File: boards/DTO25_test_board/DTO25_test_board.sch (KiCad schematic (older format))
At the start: 9 parts, among them J1 MicroFit_11, J2 Ultrafit_4, J3 Ultrafit_2, J4 Ultrafit_4

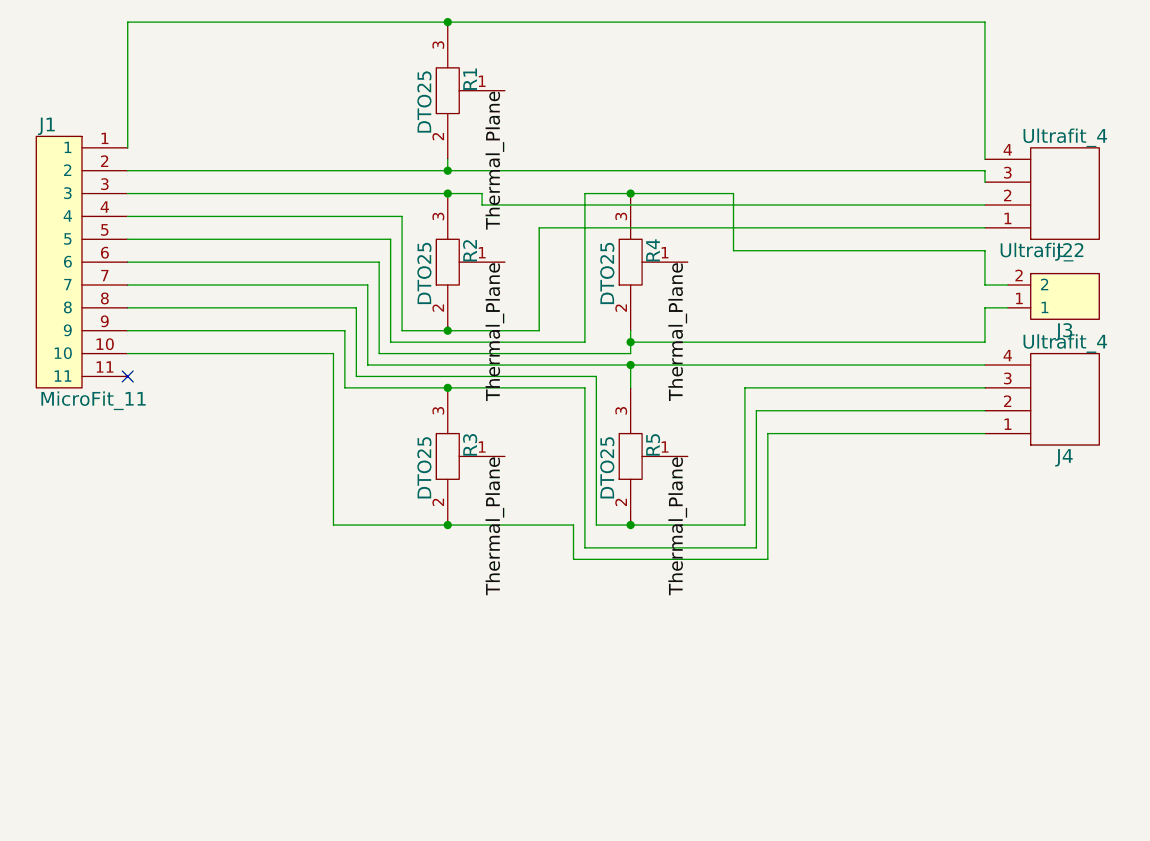
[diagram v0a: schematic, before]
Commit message: DTO@% test board MKII
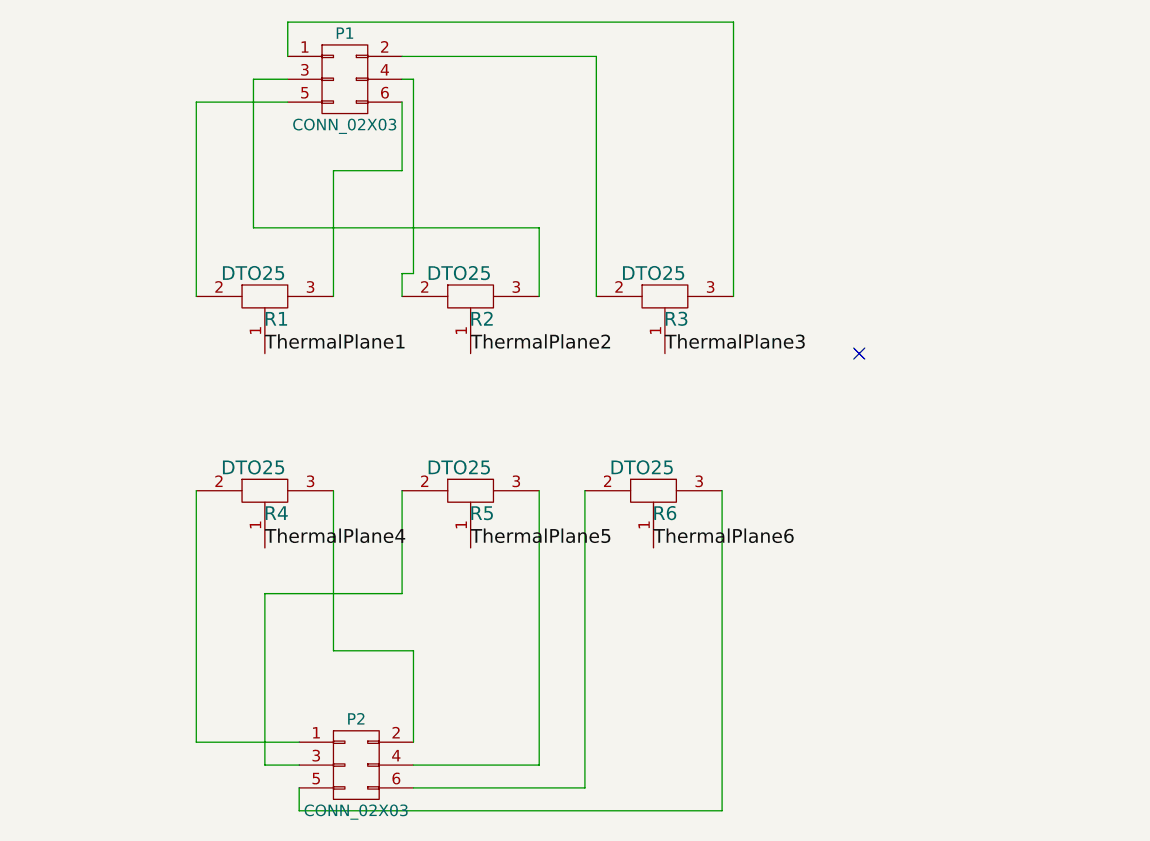
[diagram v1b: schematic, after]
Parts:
- removed J1: MicroFit_11, footprints:Molex_MicroFit_3.0-11x3.00mm_Angled, symbol MicroFit_11
- removed J2, J4: Ultrafit_4, footprints:Ultrafit_4, symbol Ultrafit_4
- removed J3: Ultrafit_2, footprints:Ultrafit_2, symbol Ultrafit_2
- added P1, P2: CONN_02X03, footprints:Pin_Header_Straight_2x03, symbol CONN_02X03
- added R6: DTO25, footprints:DTO25, symbol DTO25
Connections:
- net at R2.2: now also P1.4 (P4)
- net at R2.3: now also P1.3 (P3)
- net at R1.2: now also P1.5 (P5)
- net at R1.3: now also P1.6 (P6)
- net at R3.2: now also P1.2 (P2)
- net at R3.3: now also P1.1 (P1)
- net at R5.2: now also P2.3 (P3)
- net at R5.3: now also P2.4 (P4)
- net at R4.2: now also P2.1 (P1)
- net at R4.3: now also P2.2 (P2)
- removed net Thermal_Plane: R1.1, R2.1, R3.1, R4.1, R5.1
- new net: P2.6 (P6), R6.2
- new net: P2.5 (P5), R6.3
- new net ThermalPlane1: R1.1
- new net ThermalPlane2: R2.1
- new net ThermalPlane3: R3.1
- new net ThermalPlane4: R4.1
- new net ThermalPlane5: R5.1
- new net ThermalPlane6: R6.1
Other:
- moved on the sheet: R1, R2, R3
